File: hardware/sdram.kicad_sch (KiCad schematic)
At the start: 7 parts, among them U10 W9825G6KH

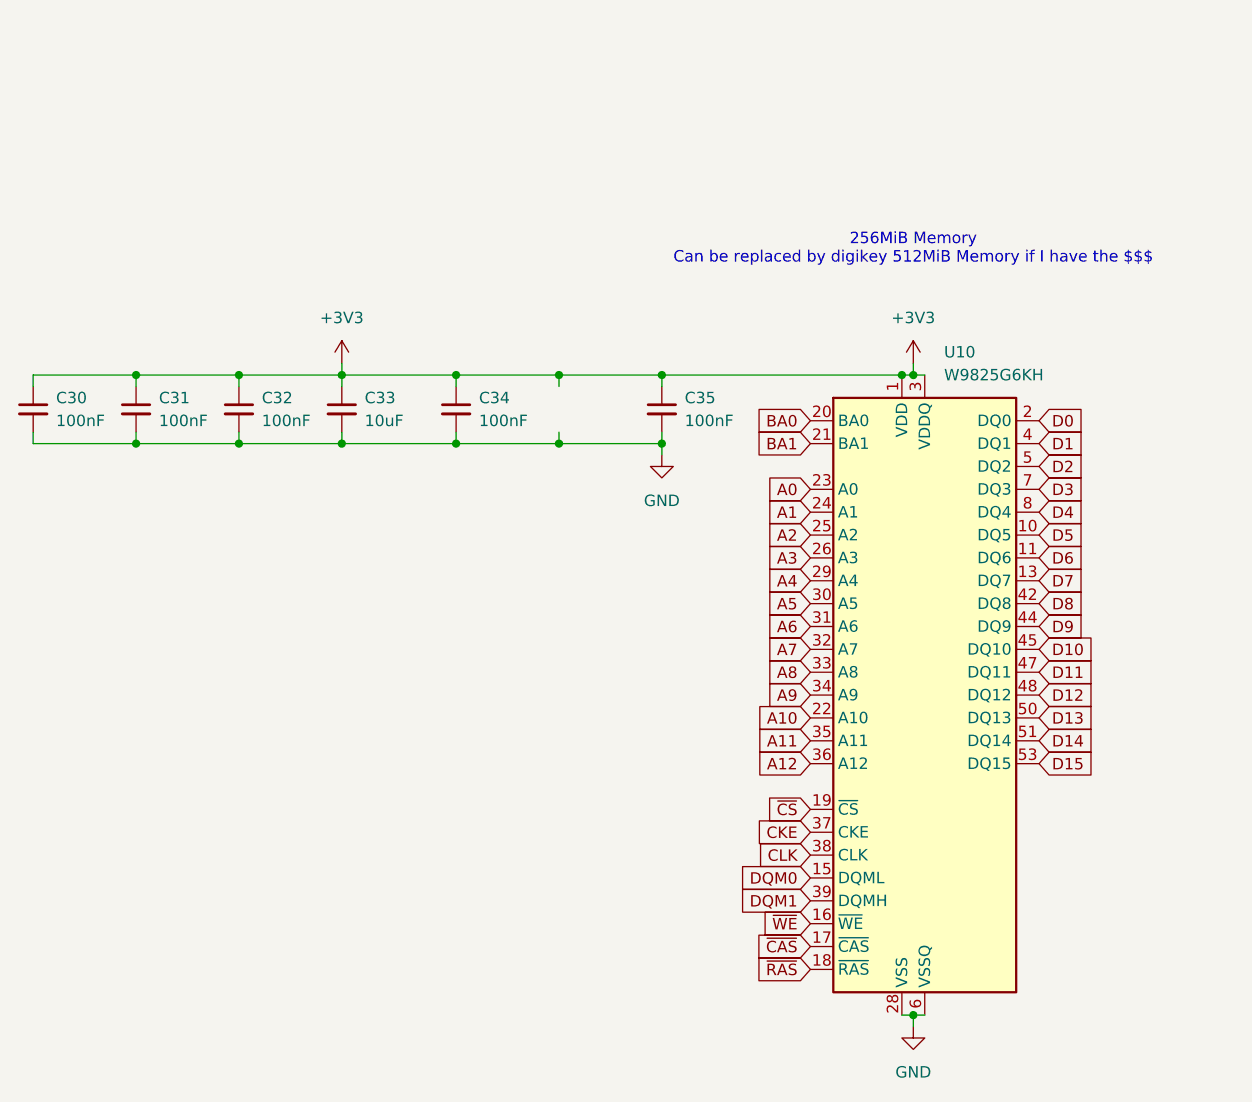
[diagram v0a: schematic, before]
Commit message: Pre-prod fixes
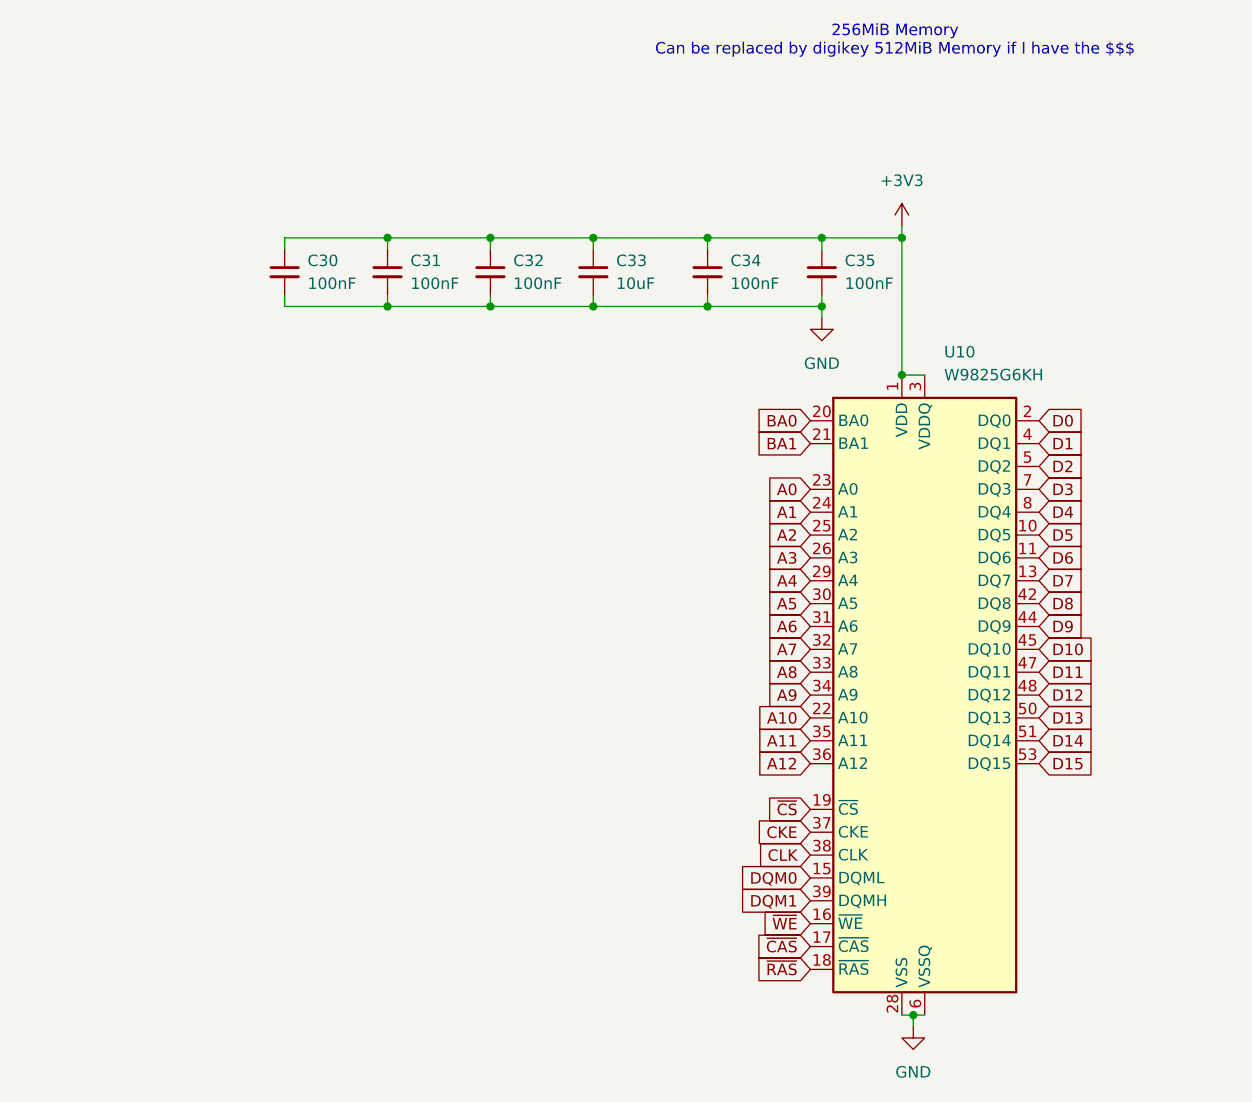
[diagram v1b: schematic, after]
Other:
- moved on the sheet: C30, C31, C32, C33, C34, C35
